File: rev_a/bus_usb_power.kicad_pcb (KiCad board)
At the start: 2 copper layers, 50 x 50 mm, 18 parts, among them J1 TERMINATE_JUMPER, Q1 FQP47P06, Q2 FQP47P06, SW1 F-426-0020

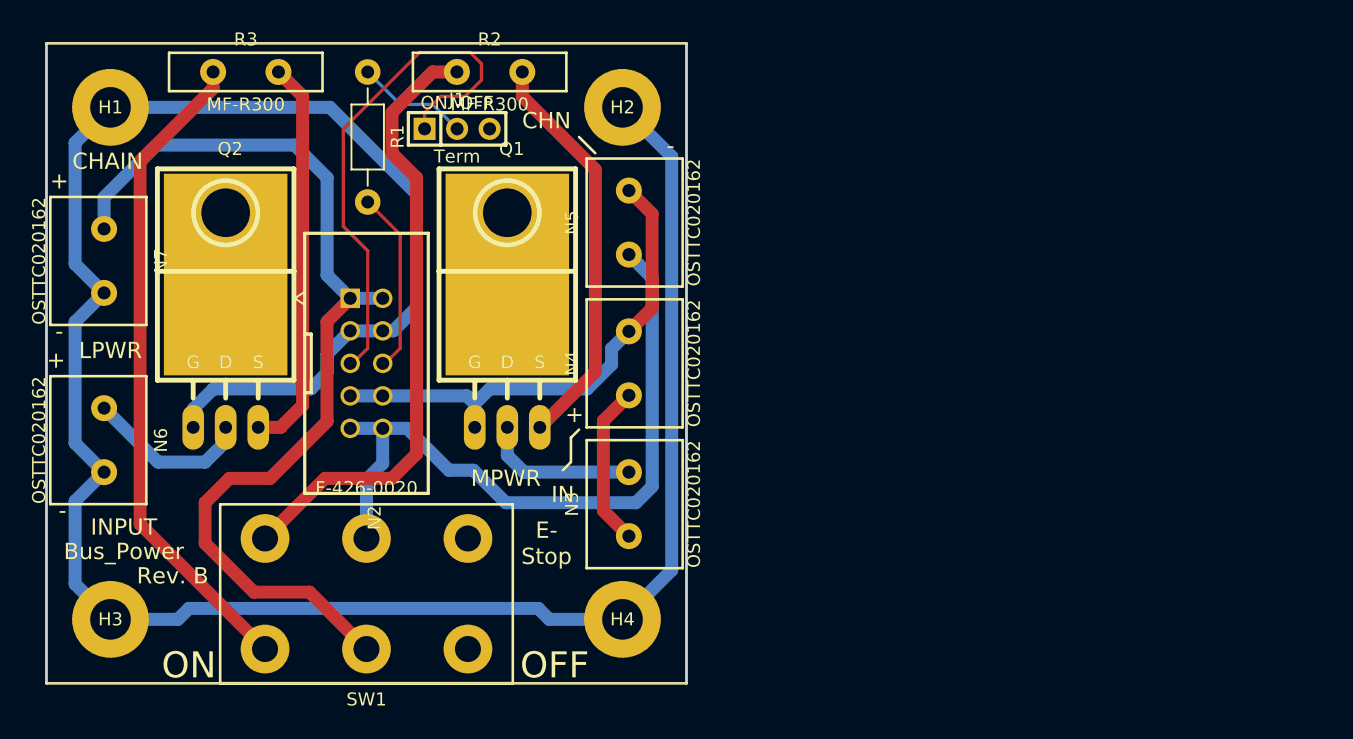
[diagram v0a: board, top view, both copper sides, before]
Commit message: Initial layout of Rev. A is complete.
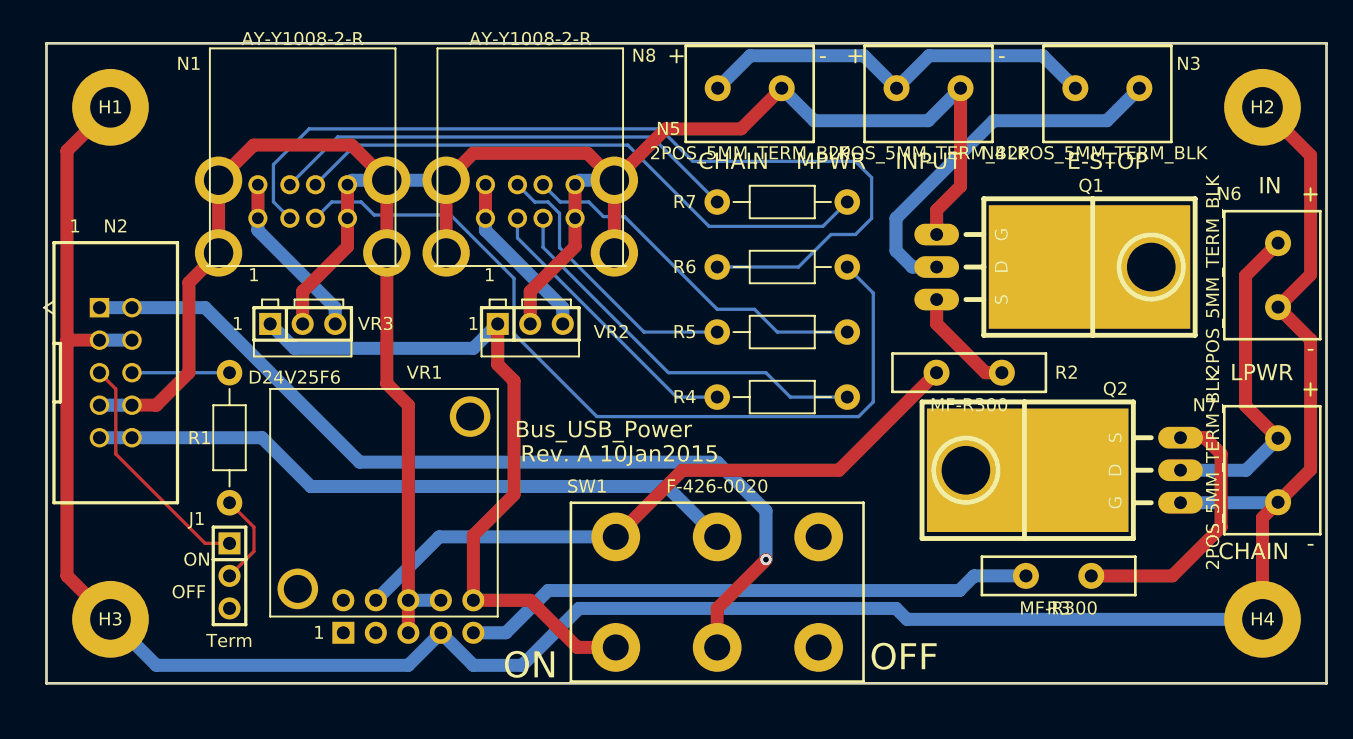
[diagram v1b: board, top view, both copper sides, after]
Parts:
- added N1: AY-Y1008-2-R, Bus_Usb_Power:DUAL_USB_A, F.Cu at (120.0, 113.7)
- added N8: AY-Y1008-2-R, Bus_Usb_Power:DUAL_USB_A, F.Cu at (137.8, 113.7)
- added R4: 200, Bus_Usb_Power:Resistor_Horizontal_400, F.Cu at (157.5, 127.6)
- added R5: 200, Bus_Usb_Power:Resistor_Horizontal_400, F.Cu at (157.5, 122.6)
- added R6: 200, Bus_Usb_Power:Resistor_Horizontal_400, F.Cu at (157.5, 117.5)
- added R7: 200, Bus_Usb_Power:Resistor_Horizontal_400, F.Cu at (157.5, 112.4)
- added VR1: D24V25F6, Bus_Usb_Power:D24V25F6, F.Cu at (126.4, 135.9)
- added VR2: OKI-78SR-5/1.5-W36-C, Bus_Usb_Power:OKI_DC_TO_DC_CONNECTOR, F.Cu at (137.8, 121.9)
- added VR3: OKI-78SR-5/1.5-W36-C, Bus_Usb_Power:OKI_DC_TO_DC_CONNECTOR, F.Cu at (120.0, 121.9)
- N3, N4, N5, N6, N7: value OSTTC020162 -> 2POS_5MM_TERM_BLK
- moved N7 93.2 mm to (196.2, 133.3)
- moved N6 92.6 mm to (196.2, 118.1)
- moved R3 74.7 mm to (179.1, 141.6)
- moved Q2 74.7 mm to (188.6, 133.3), turned to 90 degrees
- moved H2 50.0 mm to (195.0, 105.0)
- moved H4 50.0 mm to (195.0, 145.0)
- moved N3 49.5 mm to (182.9, 103.5), turned to 180 degrees
- moved R2 44.2 mm to (172.1, 125.7)
- moved J1 39.2 mm to (114.3, 141.6), turned to 270 degrees
- moved Q1 35.8 mm to (169.5, 117.5), turned to 270 degrees
- moved N4 31.8 mm to (168.9, 103.5), turned to 180 degrees
- moved SW1 27.4 mm to (152.4, 142.9)
- moved R1 25.9 mm to (114.3, 130.8), turned to 90 degrees
- moved N2 19.6 mm to (105.4, 125.7)
- moved G1 16.6 mm to (123.8, 131.4), turned to 180 degrees
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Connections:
- J1 pad 3: Net-(J1-Pad3) -> (no net)
- N2 pad 1: /LPWR4 -> /LPWR5
- N2 pad 2: /LPWR4 -> /LPWR5
- N5 pad 2: /MPWR4 -> /MPWR0
- N7 pad 2: /LPWR4 -> /LPWR1
- SW1 pad 3: Net-(SW1-Pad3) -> (no net)
- SW1 pad 4: /LPWR3 -> /LPWR4
- SW1 pad 5: /LPWR4 -> /LPWR5
- SW1 pad 6: Net-(SW1-Pad6) -> (no net)
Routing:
- net /MGND: track 39.4 -> 184.3 mm
- net Net-(N1-Pad2): track 0.00 -> 71.0 mm
- net /LPWR5: track 0.00 -> 70.9 mm, vias 0 -> 1
- net Net-(N1-Pad3): track 0.00 -> 65.4 mm
- net Net-(N1-Pad7): track 0.00 -> 46.2 mm
- net Net-(N1-Pad6): track 0.00 -> 37.0 mm
- net Net-(N8-Pad3): track 0.00 -> 30.9 mm
- net Net-(N8-Pad7): track 0.00 -> 28.5 mm
- net /MPWR2: track 31.9 -> 8.58 mm
- net Net-(J1-Pad1): track 41.5 -> 18.7 mm
- net Net-(N8-Pad2): track 0.00 -> 22.3 mm
- net Net-(N8-Pad6): track 0.00 -> 21.9 mm
- net /LPWR4: track 77.1 -> 55.4 mm
- net /MPWR0: track 12.6 -> 32.1 mm
- net /MPWR1: track 12.2 -> 29.5 mm
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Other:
- board size 50 x 50 mm -> 100 x 50 mm
- board text added: "1"
- board text added: "Bus USB Power Rev. A 10Jan2015 (c) Gramlich"
- board text added: "Bus_USB_Power"
- board text added: "E-STOP"
- board text added: "Rev. A 10Jan2015"
- board text removed: "Bus Power Rev. B 1Oct2014 (c) Gramlich"
- board text removed: "Bus_Power"
- board text removed: "CHN"
- board text removed: "E- Stop"
- board text removed: "ON OFF"
- board text removed: "Rev. B"
